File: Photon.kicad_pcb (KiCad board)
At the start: 2 copper layers, 22.4 x 95.8 mm, 58 parts, among them J1 USB_C_Receptacle_USB2.0_14P, Q1 IRLML6402, Q2 IRLML6402, SW1 TS-1088-AR02016, U1 ATtiny13A-S, U2 RT8059GJ5, U3 TP4056, U4 BCR421UW6-7, U5 DW01A, U6 FS8205A, U7 BCR421UW6-7

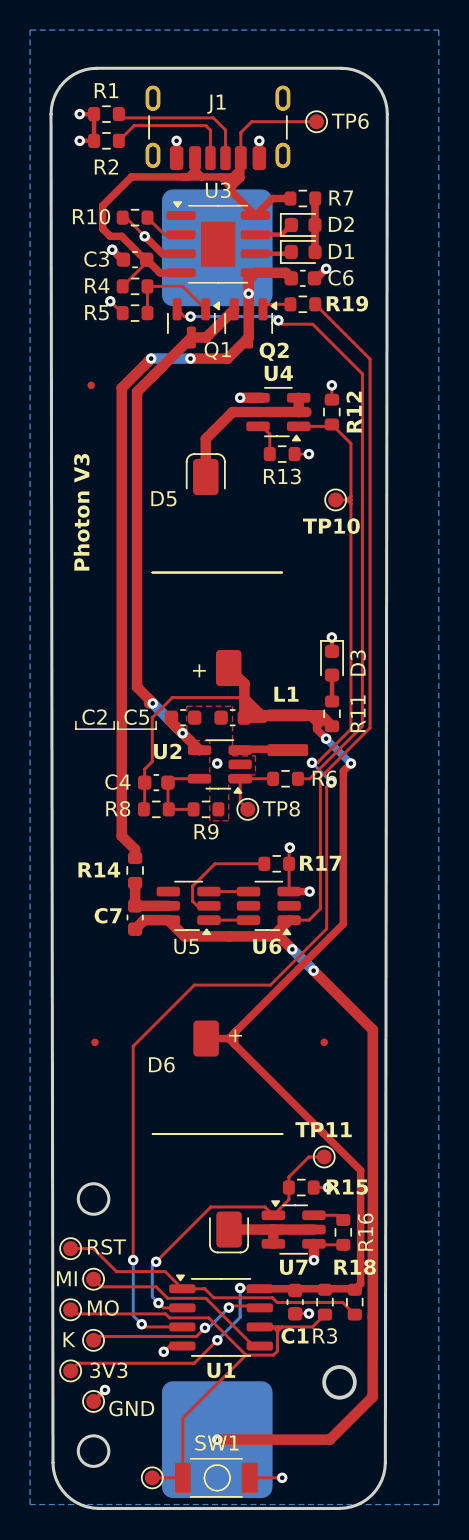
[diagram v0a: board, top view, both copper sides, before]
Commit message: Cleaned up PCB
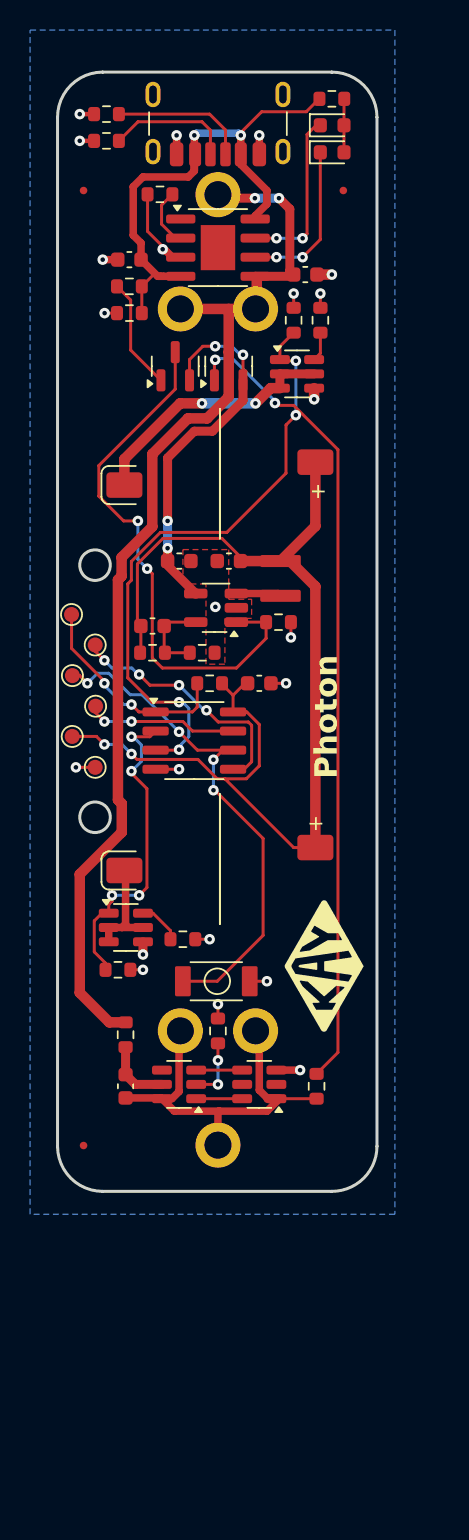
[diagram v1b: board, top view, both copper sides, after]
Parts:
- removed D3: SZYY0603R1, LED_SMD:LED_0603_1608Metric
- removed R11: 300, Resistor_SMD:R_0603_1608Metric
- removed R3: 100K, Resistor_SMD:R_0603_1608Metric
- removed TP10: LED1_EN, TestPoint:TestPoint_Pad_D1.0mm
- removed TP11: LED2_EN, TestPoint:TestPoint_Pad_D1.0mm
- removed TP2: MOSI, TestPoint:TestPoint_Pad_D1.0mm
- removed TP3: RESET, TestPoint:TestPoint_Pad_D1.0mm
- removed TP4: MISO, TestPoint:TestPoint_Pad_D1.0mm
- removed TP5: SCK, TestPoint:TestPoint_Pad_D1.0mm
- removed TP6: 5V, TestPoint:TestPoint_Pad_D1.0mm
- added G***: LOGO, Photon:KAY Logo 10x10mm, F.Cu at (59.9, 79.8)
- added G***: LOGO, Photon:KAY Logo 10x10mm, B.Cu at (52.8, 51.1)
- added TP12: SCK, TestPoint:TestPoint_Pad_D1.0mm, F.Cu at (44.7, 62.5)
- added TP13: RESET, TestPoint:TestPoint_Pad_D1.0mm, F.Cu at (43.1, 56.4)
- BT1: footprint Photon:18650 Battery Holder -> Photon:Spring Battery TH
- R4: value 10K -> 100R
- R6: value 0R -> 100K
- TP7: value BTN -> MOSI
- TP8: value BuckEN -> MISO
- U4, U5, U6, U7: footprint Package_TO_SOT_SMD:SOT-23-6_Handsoldering -> Package_TO_SOT_SMD:SOT-23-6
- moved FID3 56.6 mm to (43.9, 28.2)
- moved TP7 55.5 mm to (44.7, 58.4), turned to -90 degrees
- moved R19 52.0 mm to (59.4, 87.8), turned to 90 degrees
- moved R18 42.3 mm to (52.3, 61.0), turned to 180 degrees
- moved TP9 42.2 mm to (43.2, 64.5)
- moved TP1 42.2 mm to (44.7, 66.5)
- moved C1 41.2 mm to (55.6, 61.0), turned to 180 degrees
- moved U1 38.4 mm to (51.3, 64.8)
- moved SW1 33.0 mm to (52.8, 80.8)
- moved U7 23.0 mm to (46.8, 77.2)
- moved R16 22.2 mm to (50.5, 78.0), turned to 0 degrees
- moved FID1 21.2 mm to (61.2, 28.2)
- moved R15 18.9 mm to (46.2, 80.0)
- moved D6 18.3 mm to (53.0, 72.6), turned to 180 degrees
- moved FID2 17.4 mm to (43.9, 91.7)
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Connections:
- C2 pad 2: PACK_Safe -> PACK_SAFE
- Q1 pad 1: /USB_DSBL -> /DSBL
- Q1 pad 2: /PMOS_EN_OUT -> PACK_SAFE
- Q1 pad 3: PACK_Safe -> /BUCK_EN
- Q2 pad 2: PACK_Safe -> PACK_SAFE
- R4 pad 1: 5V -> /DSBL
- R4 pad 2: /USB_DSBL -> 5V
- R5 pad 1: /USB_DSBL -> 5V
- R6 pad 2: /PMOS_EN_OUT -> GND
- TP7 pad 1: /MISO_BTN -> /MOSI
- TP8 pad 1: /BUCK_EN -> /MISO_BTN
- U2 pad 4: PACK_Safe -> PACK_SAFE
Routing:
- net /Bat-: track 102.0 -> 26.9 mm, vias 3 -> 0
- net /BAT_DSBL: track 1.96 -> 54.3 mm, vias 0 -> 2
- net /PMOS_EN_OUT: track 43.3 -> 0.00 mm, vias 2 -> 0
- net /LED1_EN: track 77.6 -> 41.4 mm
- net PACK_Safe: track 35.6 -> 0.00 mm, vias 2 -> 0
- net /BUCK_EN: track 4.45 -> 36.4 mm, vias 0 -> 2
- net /Bat+: track 48.5 -> 73.6 mm, vias 3 -> 2
- net PACK_SAFE: track 0.00 -> 24.6 mm, vias 0 -> 4
- net +3V3: track 97.4 -> 74.5 mm, vias 4 -> 2
- net /STAT1: track 2.65 -> 11.3 mm, vias 0 -> 2
- net /STAT2: track 2.44 -> 11.0 mm, vias 0 -> 2
- net /DSBL: track 0.00 -> 7.46 mm
- net /OUT_LED1: track 10.7 -> 17.3 mm, vias 0 -> 2
- net /USB_DSBL: track 6.49 -> 0.00 mm
- net /RESET: track 20.7 -> 14.4 mm, vias 0 -> 2
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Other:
- board size 22.4 x 95.8 mm -> 21.2 x 74.4 mm
- board text added: "Photon"
- board text removed: "3V3"
- board text removed: "GND"
- board text removed: "K"
- board text removed: "MI"
- board text removed: "MO"
- board text removed: "Photon V3"
- board text removed: "RST"
